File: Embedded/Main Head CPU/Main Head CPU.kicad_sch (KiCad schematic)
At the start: 47 parts, among them J1 10171746-00021LF, J10 Fan 1, J11 Substructure Power, J12 Head Power, J13 MicroSD, J2 Maw, J3 Tongue, J4 Left Fin, J5 Right Fin, J6 Scales, J7 Extra, J8 Conn_01x06, J9 Fan 0, Q1 DMG3402L, Q2 DMG3402L, SW1 Boot, SW2 RST, U1 Sensored, U2 Buttons, U3 LD1117S33TR_SOT223, U4 LD1117S50TR_SOT223, U5 Substructure

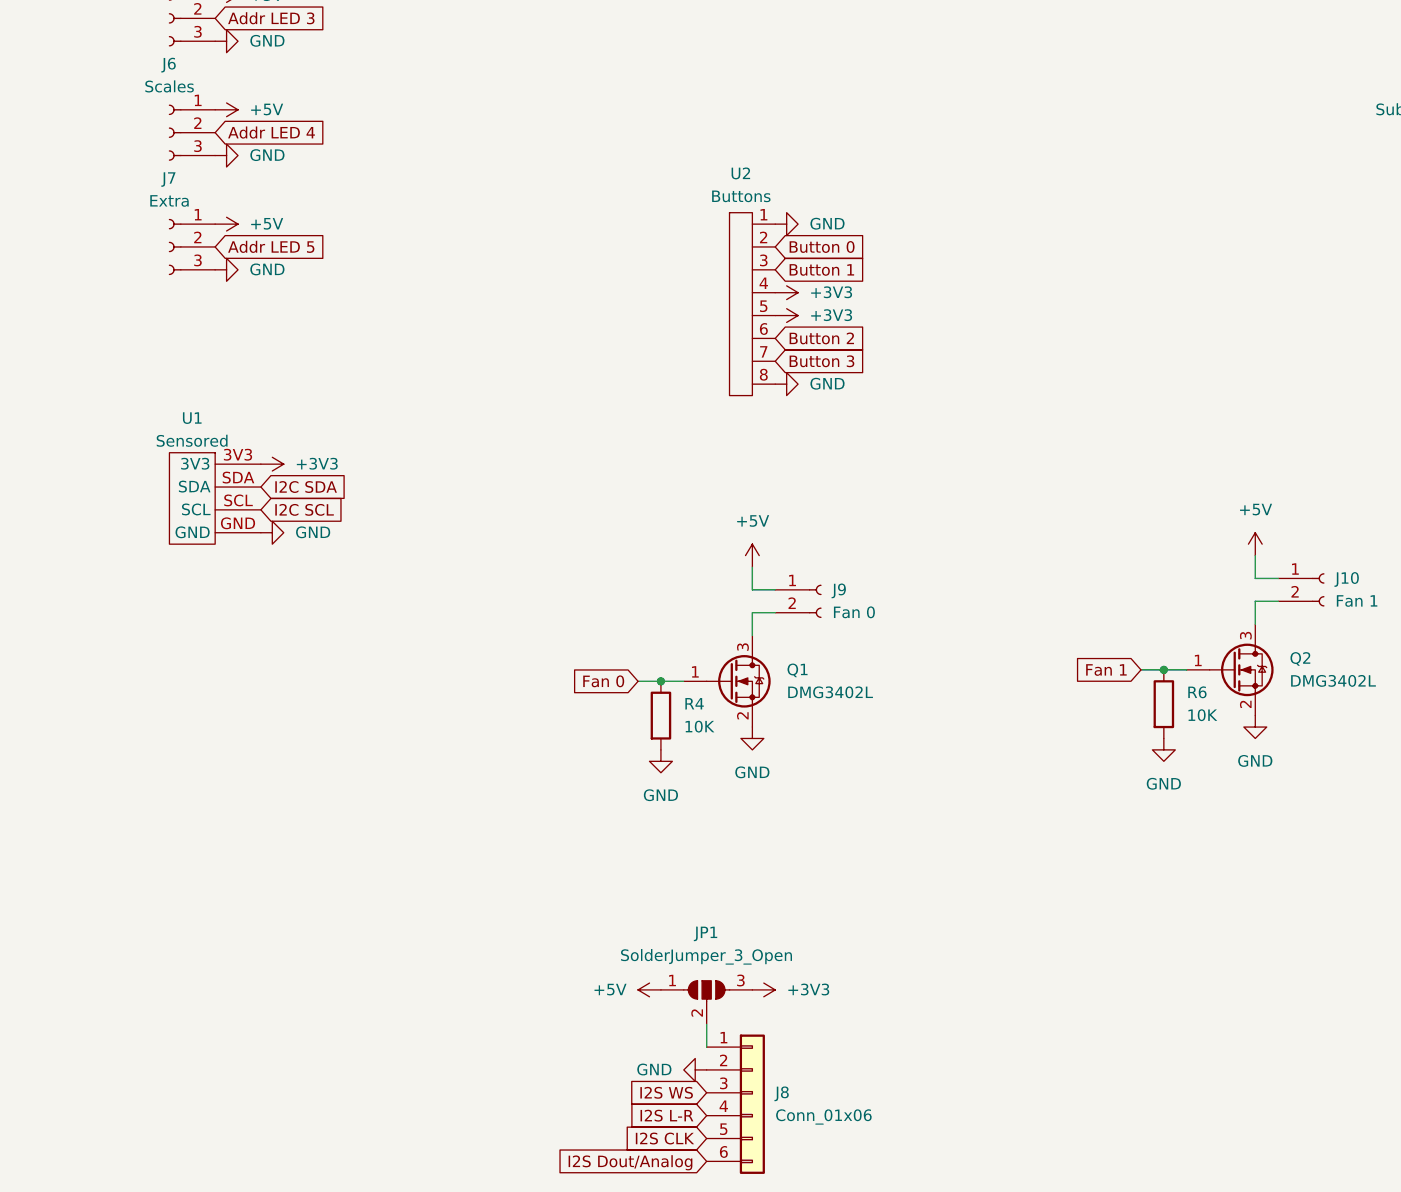
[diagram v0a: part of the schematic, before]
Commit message: Modified Routing & Silkscreen
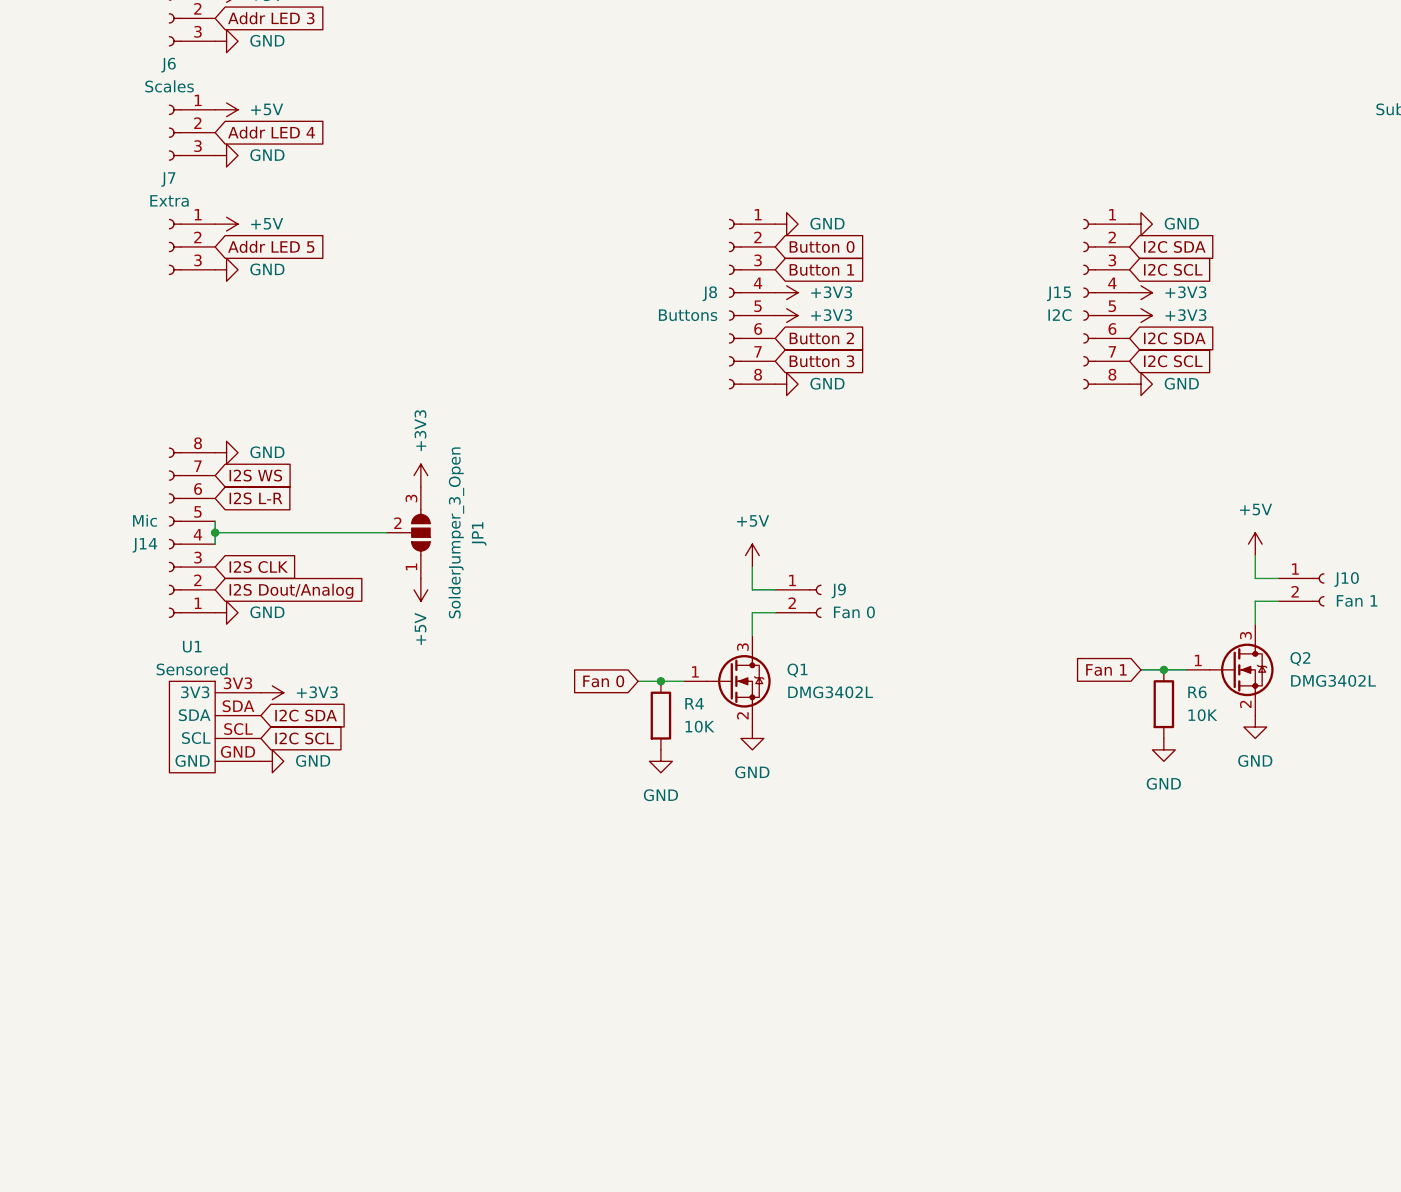
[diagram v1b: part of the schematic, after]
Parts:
- removed J8: Conn_01x06, Connector_PinHeader_2.54mm:PinHeader_1x06_P2.54mm_Vertical, symbol Connector_Generic:Conn_01x06
- removed U2: Buttons, FCC:FFC 0.8mm 8P, symbol FFC:FFC-8
- added J14: Mic, Connector_JST:JST_GH_SM08B-GHS-TB_1x08-1MP_P1.25mm_Horizontal, symbol Connector:Conn_01x08_Socket
- added J15: I2C, Connector_JST:JST_GH_SM08B-GHS-TB_1x08-1MP_P1.25mm_Horizontal, symbol Connector:Conn_01x08_Socket
- added J8: Buttons, Connector_JST:JST_GH_SM08B-GHS-TB_1x08-1MP_P1.25mm_Horizontal, symbol Connector:Conn_01x08_Socket
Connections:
- net +3V3: now also J15.4 (Pin_4), J15.5 (Pin_5), J8.4 (Pin_4), J8.5 (Pin_5)
- net Button 0: now also J8.2 (Pin_2)
- net Button 1: now also J8.3 (Pin_3)
- net Button 2: now also J8.6 (Pin_6)
- net Button 3: now also J8.7 (Pin_7)
- net GND: now also J14.1 (Pin_1), J14.8 (Pin_8), J15.1 (Pin_1), J15.8 (Pin_8), J8.1 (Pin_1), J8.8 (Pin_8)
- net I2C SCL: now also J15.3 (Pin_3), J15.7 (Pin_7)
- net I2C SDA: now also J15.2 (Pin_2), J15.6 (Pin_6)
- net I2S CLK: now also J14.3 (Pin_3)
- net I2S Dout/Analog: now also J14.2 (Pin_2)
- net I2S L-R: now also J14.6 (Pin_6)
- net I2S WS: now also J14.7 (Pin_7)
- net at JP1.2 (C): now also J14.4 (Pin_4), J14.5 (Pin_5)
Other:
- moved on the sheet: JP1, U1
